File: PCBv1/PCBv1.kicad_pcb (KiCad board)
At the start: 2 copper layers, 30 x 40 mm, 8 parts

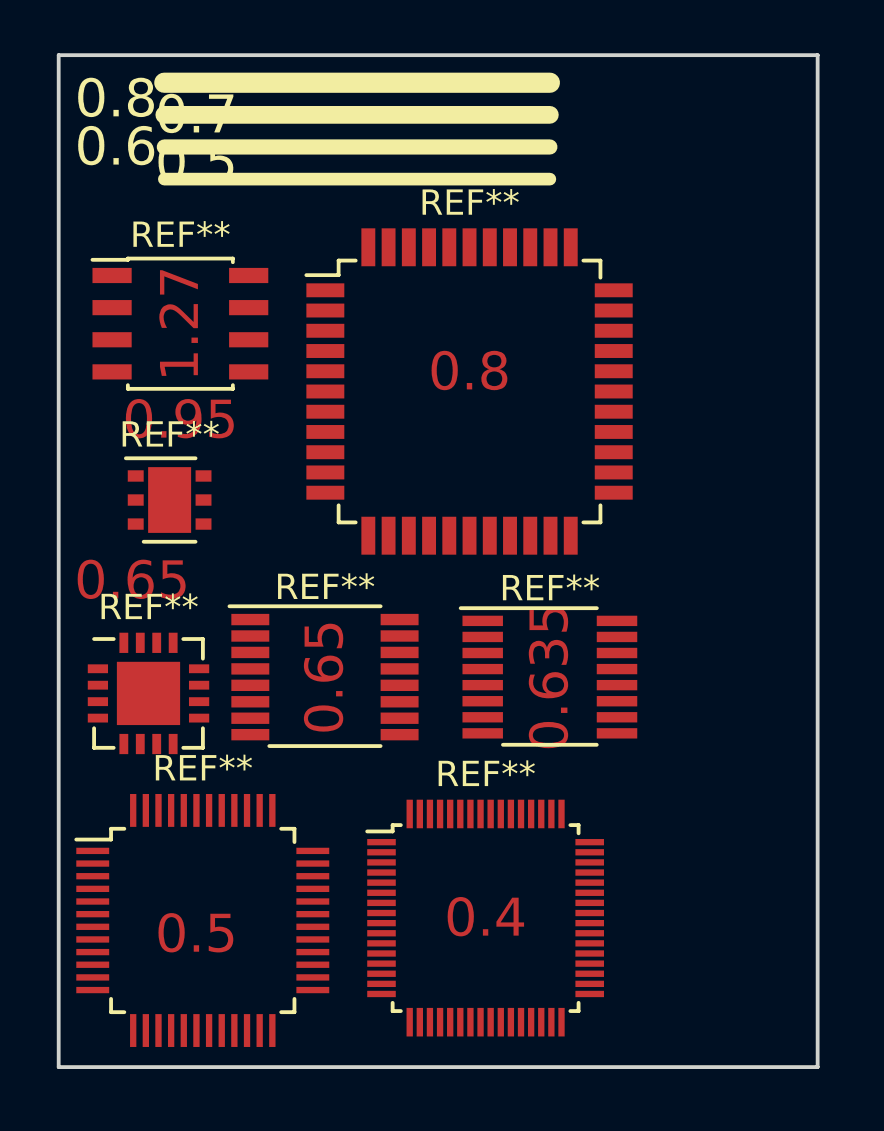
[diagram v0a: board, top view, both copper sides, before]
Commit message: Completed v1 PCB
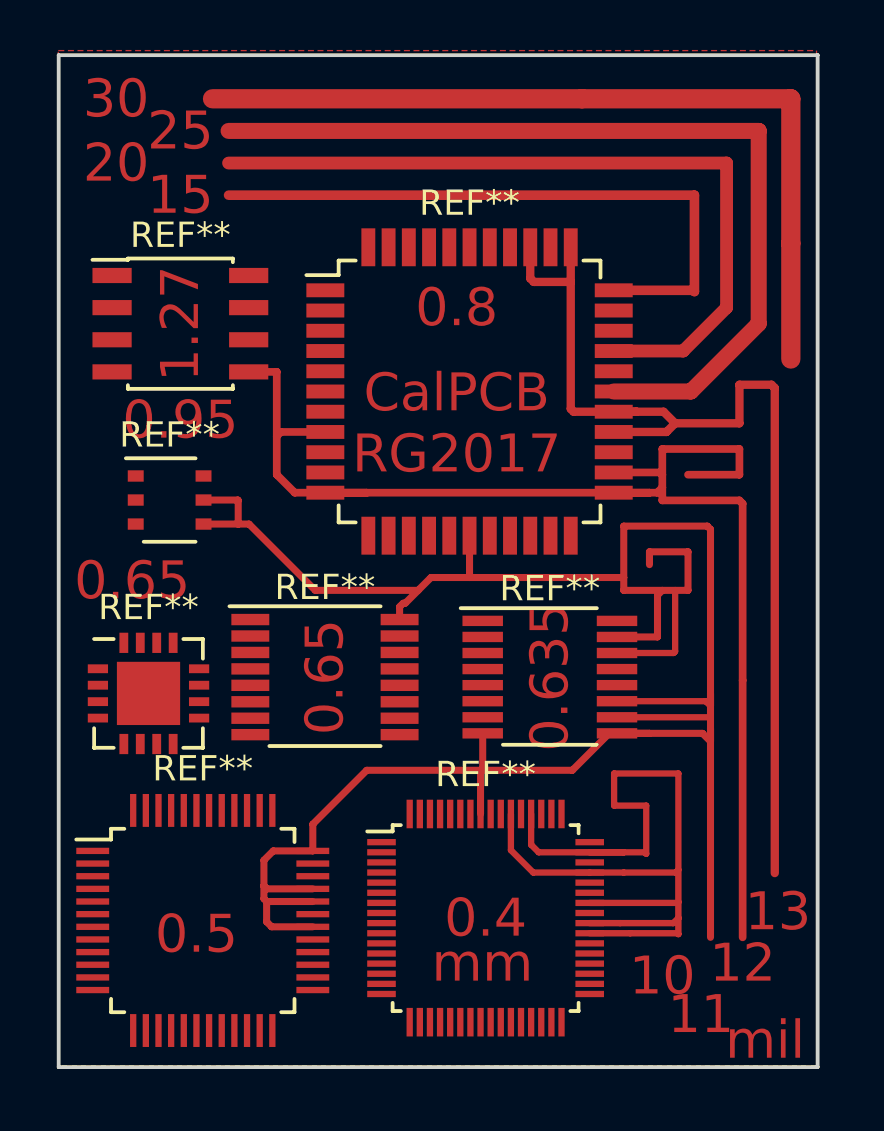
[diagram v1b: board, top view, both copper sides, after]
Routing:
- net (no net): track 0.00 -> 363.9 mm
- added copper zone on F.Cu, net (none)
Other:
- board text added: "10"
- board text added: "11"
- board text added: "12"
- board text added: "13"
- board text added: "15"
- board text added: "20"
- board text added: "25"
- board text added: "30"
- board text added: "CalPCB RG2017"
- board text added: "mil"
- board text added: "mm"
- board text removed: "0.6"
- board text removed: "0.7"
